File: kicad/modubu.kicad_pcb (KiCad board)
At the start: 2 copper layers, 100 x 92 mm, 45 parts, among them J1 AudioJack4, J2 AudioJack4, SW1 SW_Push, SW10 SW_Push, SW11 SW_Push, SW12 SW_Push, SW13 SW_Push, SW14 SW_Push, SW15 SW_Push, SW16 SW_Push, SW17 SW_Push, SW18 SW_Push, SW19 SW_Push, SW2 SW_Push, SW3 SW_Push, SW4 SW_Push, SW5 SW_Push, SW6 SW_Push, SW7 SW_Push, SW8 SW_Push, SW9 SW_Push, U1 RP2040-Zero

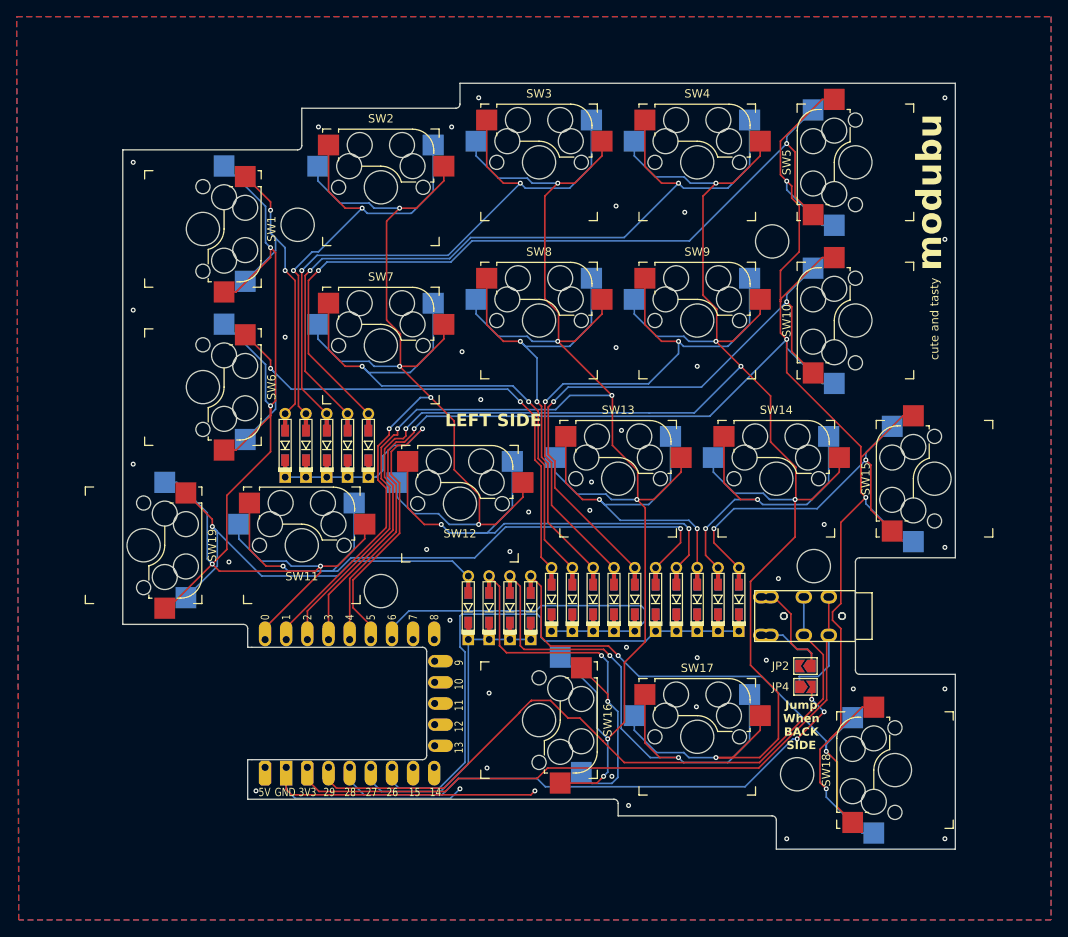
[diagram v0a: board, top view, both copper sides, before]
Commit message: add board art
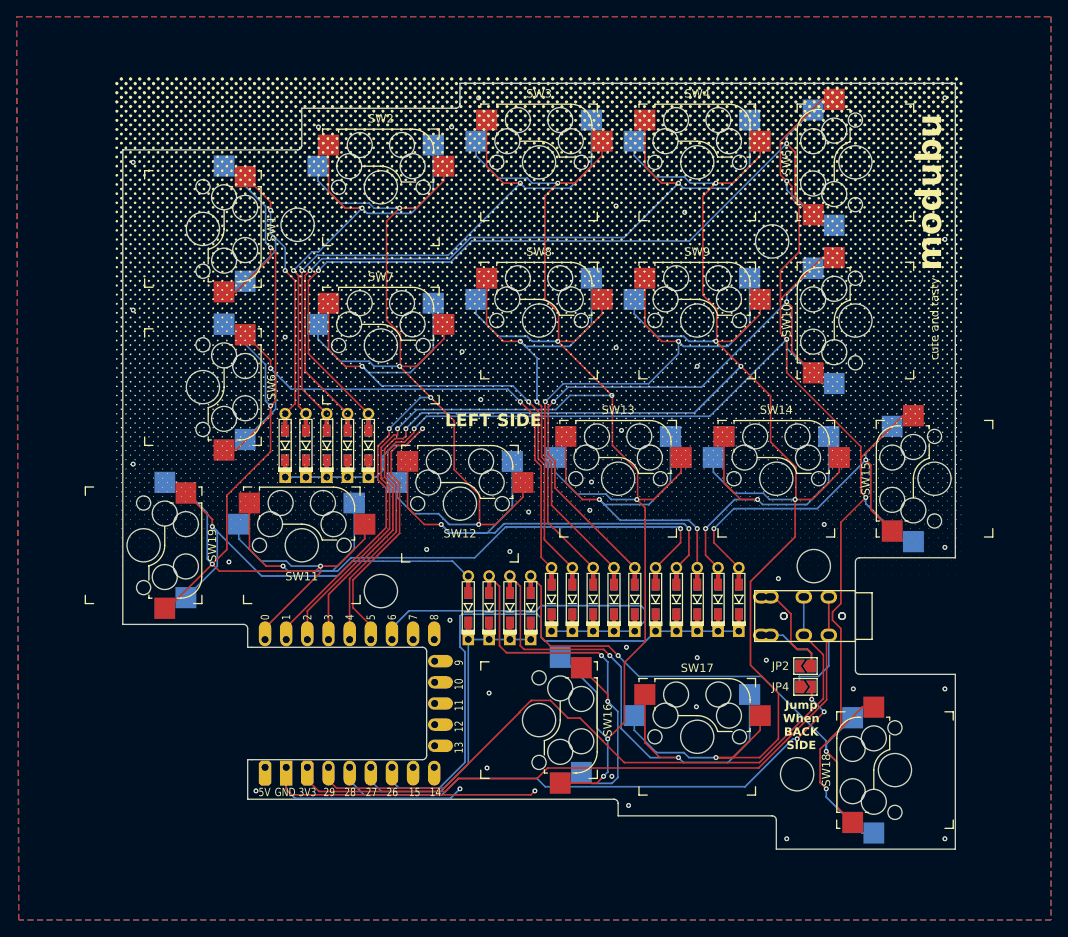
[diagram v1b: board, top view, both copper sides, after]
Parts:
- added G***: LOGO, modubu-CustomFoot:meshgradation, F.Cu at (90.5, 100.5)
- added G***: LOGO, modubu-CustomFoot:meshgradation, B.Cu at (90.5, 100.5)
